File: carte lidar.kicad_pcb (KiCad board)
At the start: 2 copper layers, 40 x 40 mm, 33 parts, among them J1 UART CP, J2 LIDAR, J3 XBEE, J8 alim, U1 XIAO-ESP32-S3-DIP

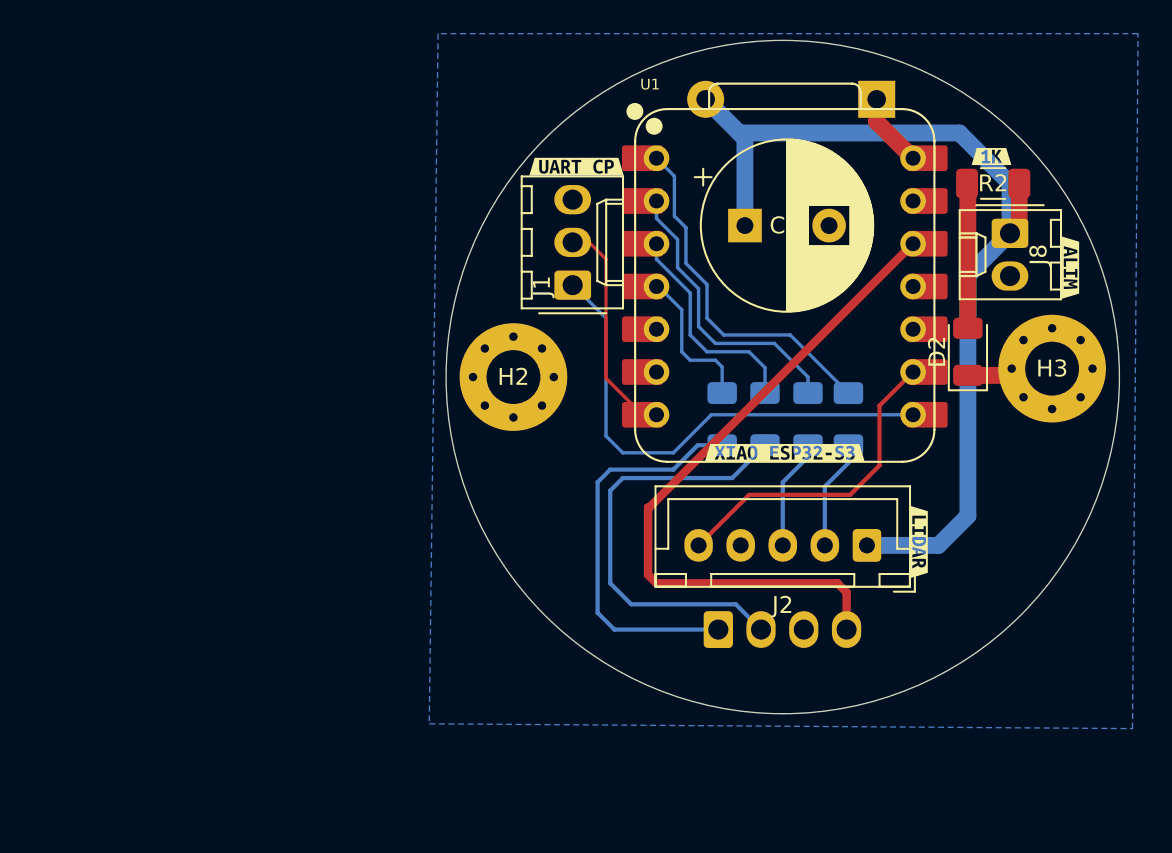
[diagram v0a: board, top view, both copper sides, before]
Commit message: v2 un poil violent XD
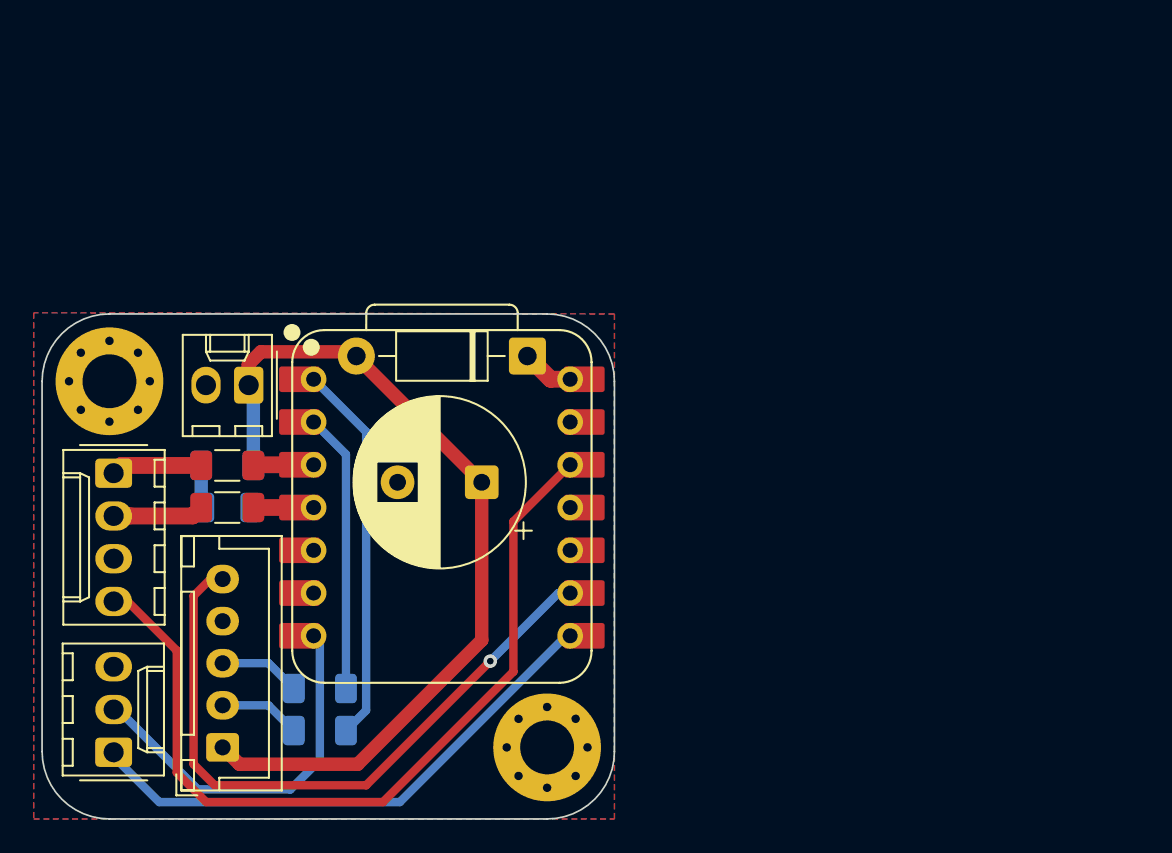
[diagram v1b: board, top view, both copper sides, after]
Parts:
- removed kibuzzard-67ED5E55 (x2): G***, kibuzzard-67ED5E55
- removed kibuzzard-67ED8412: G***, kibuzzard-67ED8412
- removed kibuzzard-67ED8456: G***, kibuzzard-67ED8456
- removed kibuzzard-68F1EF6D: G***, kibuzzard-68F1EF6D
- removed kibuzzard-68F1EFC1: G***, kibuzzard-68F1EFC1
- removed kibuzzard-68F1EFDA: G***, kibuzzard-68F1EFDA
- removed kibuzzard-68F1EFE5: G***, kibuzzard-68F1EFE5
- removed kibuzzard-68F1F041: G***, kibuzzard-68F1F041
- removed kibuzzard-68F1F0CD: G***, kibuzzard-68F1F0CD
- removed kibuzzard-68F1F1A3: G***, kibuzzard-68F1F1A3
- removed kibuzzard-68F1F1EA: G***, kibuzzard-68F1F1EA
- removed kibuzzard-68F1F1F6: G***, kibuzzard-68F1F1F6
- removed kibuzzard-68F1F236: G***, kibuzzard-68F1F236
- removed kibuzzard-68F1F243: G***, kibuzzard-68F1F243
- removed kibuzzard-68F1F26D: G***, kibuzzard-68F1F26D
- removed kibuzzard-68F1F2E0: G***, kibuzzard-68F1F2E0
- removed kibuzzard-68F1F3B3: G***, kibuzzard-68F1F3B3
- D1, J3, R4, R5: moved to F.Cu
- D2, R2: moved to B.Cu
- moved R2 48.5 mm to (107.0, 55.2)
- moved J8 46.1 mm to (108.3, 50.5), turned to 180 degrees
- moved D2 45.0 mm to (107.0, 57.8), turned to 180 degrees
- moved J2 40.1 mm to (106.7, 72.0), turned to 90 degrees
- moved J1 38.9 mm to (100.2, 72.3)
- moved H3 37.5 mm to (126.0, 72.0)
- moved J3 37.1 mm to (100.2, 55.7), turned to -90 degrees
- moved R1 36.4 mm to (112.5, 71.0), turned to 0 degrees
- moved R3 33.1 mm to (112.5, 68.5), turned to 0 degrees
- moved R4 32.1 mm to (107.0, 55.2), turned to 0 degrees
- moved R5 29.9 mm to (107.0, 57.8), turned to 0 degrees
- moved D1 25.8 mm to (124.8, 48.8)
- moved U1 24.2 mm to (119.8, 57.8)
- moved H2 24.0 mm to (100.0, 50.2)
- moved C1 21.8 mm to (122.1, 56.2), turned to 180 degrees
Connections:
- R4 pad 1: TX XBEE -> RX XBEE
- R5 pad 1: RX XBEE -> TX XBEE
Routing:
- net Lidar_PWM: track 19.1 -> 39.8 mm, vias 0 -> 1
- net TX XBEE: track 25.9 -> 6.41 mm
- net RX XBEE: track 23.6 -> 5.39 mm
- net +3.3V: track 40.7 -> 50.7 mm
- net UART CPS: track 12.5 -> 22.4 mm
- net Net-(U1-GPIO3/D2/A2): track 13.0 -> 3.60 mm
- net Net-(D2-A): track 8.62 -> 2.56 mm
- net Net-(U1-GPIO4/D3/A3): track 8.89 -> 3.58 mm
- net +5V: track 56.5 -> 51.8 mm
- net UART CPE: track 29.4 -> 32.3 mm
- net GND: track 2.77 -> 0.00 mm
- net RX LIDAR: track 6.57 -> 4.85 mm
- net TX LIDAR: track 6.53 -> 4.85 mm
- net Net-(U1-GPIO1/D0/A0): track 21.0 -> 22.7 mm
- net Net-(D1-K): track 4.39 -> 3.11 mm
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- added copper zone on F.Cu, net GND
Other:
- board size 40 x 40 mm -> 34 x 30 mm
